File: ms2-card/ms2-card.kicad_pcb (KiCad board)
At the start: 2 copper layers, 100 x 54 mm, 30 parts, among them J10 MicroSD_SPI_CD, J11 I2C, J20 Smartcard Connector, J21 Card Edge, J22 Card Edge, J23 Conn_01x04, J30 Power_Only, M1 PI_PICO_ZERO, Q30 BC847, SW1 SW_Push, U1 W25Q128JVS

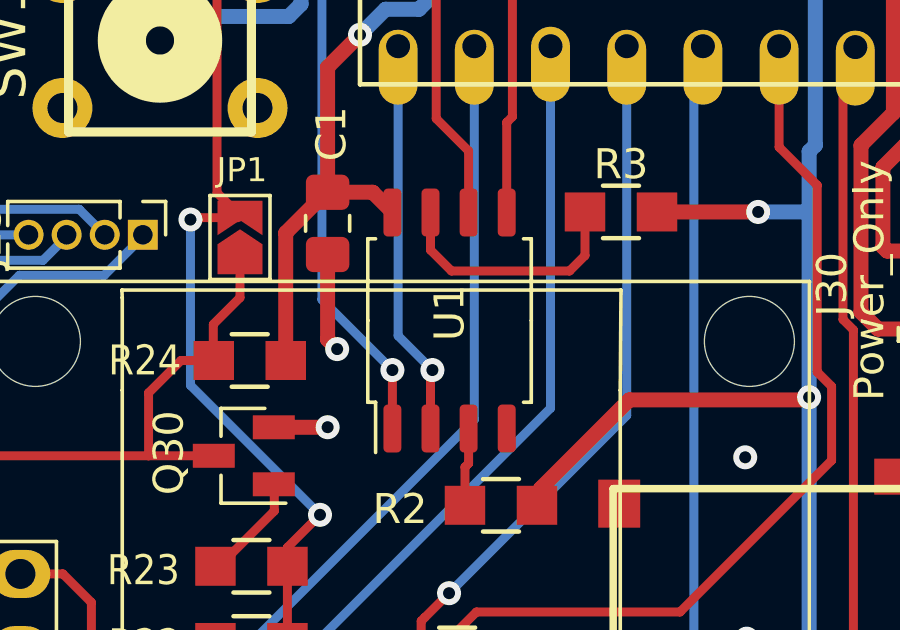
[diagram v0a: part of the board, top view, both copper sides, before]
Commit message: modified ground a little bit
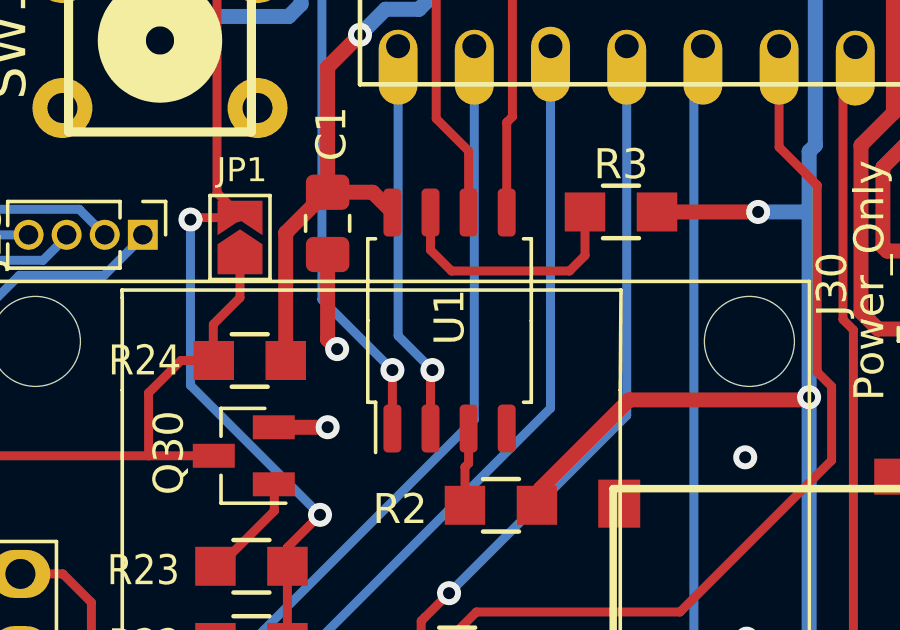
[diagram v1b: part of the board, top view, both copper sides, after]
